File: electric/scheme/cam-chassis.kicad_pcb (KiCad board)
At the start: 2 copper layers, 51.5 x 28.5 mm, 48 parts, among them IC1 ATMEGA8-AI, K1 pyro, P1 TST, P2 TST, P3 TST, P4 TST, P5 TST, P6 TST, P7 servo, Q3 bc857, Q4 bc847, Q5 irlml2244, Q6 NPN, Q7 irlml2244, U1 MINI-USB-B-4-bases, Y1 Crystal

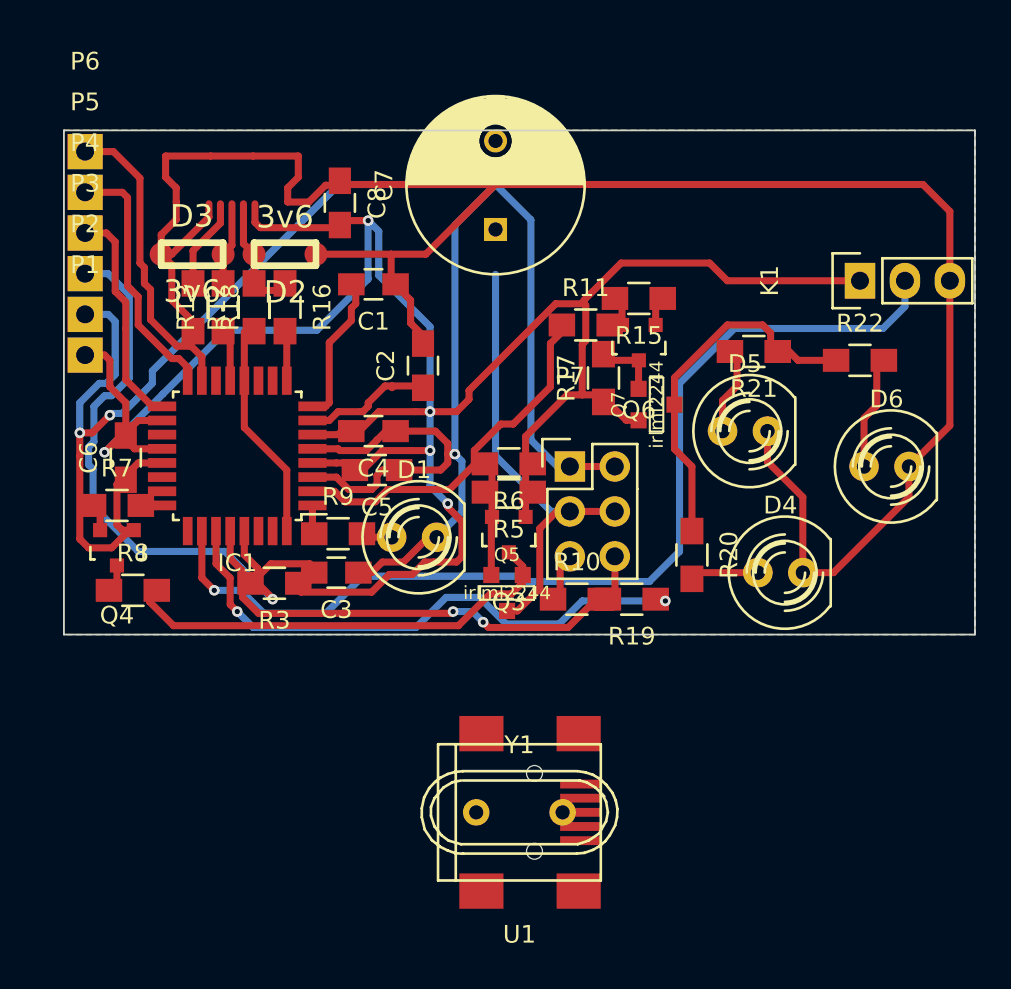
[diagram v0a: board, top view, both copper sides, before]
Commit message: a
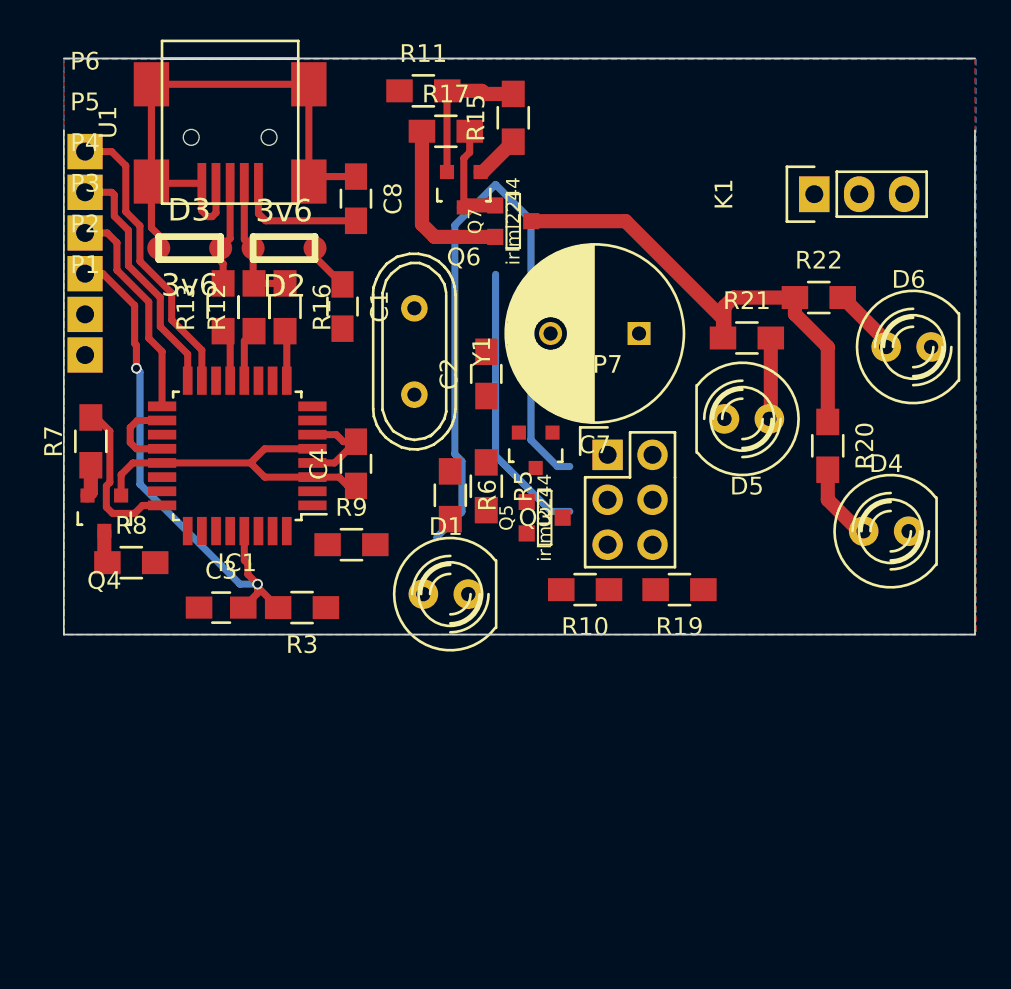
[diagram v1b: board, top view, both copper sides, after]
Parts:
- removed C5, C6: 100n, Capacitors_SMD:C_0805_HandSoldering
- removed R18: 100k, Resistors_SMD:R_0805_HandSoldering
- moved U1 42.3 mm to (107.9, 83.5), turned to 270 degrees
- moved Y1 26.7 mm to (118.3, 96.5), turned to 270 degrees
- moved R17 16.6 mm to (120.1, 84.1), turned to 0 degrees
- moved R11 16.1 mm to (118.8, 81.8)
- moved Q7 13.2 mm to (123.9, 89.1)
- moved Q6 13.1 mm to (121.1, 87.4)
- moved R15 12.4 mm to (123.9, 83.3), turned to 90 degrees
- moved C7 10.0 mm to (131.0, 95.5), turned to 180 degrees
- moved R20 9.85 mm to (141.7, 101.8)
- moved D6 6.87 mm to (146.3, 96.2)
- moved C3 6.80 mm to (107.4, 111.0), turned to 0 degrees
- moved D4 6.42 mm to (145.0, 106.7)
- moved K1 5.53 mm to (140.9, 87.6)
- moved Q3 5.00 mm to (125.2, 102.1)
- moved Q5 4.76 mm to (125.7, 105.9), turned to 90 degrees
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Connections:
- U1 pad 4: Net-(R18-Pad1) -> GND
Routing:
- net GND: track 239.9 -> 58.1 mm, vias 3 -> 0
- net VCC: track 135.7 -> 27.4 mm, vias 5 -> 0
- net /pyro-sen: track 57.7 -> 0.00 mm, vias 1 -> 0
- net (no net): track 0.00 -> 55.5 mm
- net /servo1: track 32.5 -> 0.00 mm, vias 2 -> 0
- net /servo2: track 25.4 -> 0.00 mm, vias 2 -> 0
- net /gate: track 25.3 -> 0.00 mm
- net /servo-vcc: track 21.0 -> 0.00 mm
- net /led: track 14.5 -> 0.00 mm
- net /src: track 12.6 -> 0.00 mm
- net /d-: track 13.0 -> 3.13 mm
- net /xtal2: track 8.35 -> 0.00 mm
- net /rst: track 37.4 -> 29.5 mm, vias 1 -> 2
- net Net-(P7-Pad5): track 7.84 -> 0.00 mm
- net /xtal1: track 7.34 -> 0.00 mm
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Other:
- board size 51.5 x 28.5 mm -> 51.5 x 32.6 mm
